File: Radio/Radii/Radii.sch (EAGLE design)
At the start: 14 parts, among them U2 LEV_SHIFT

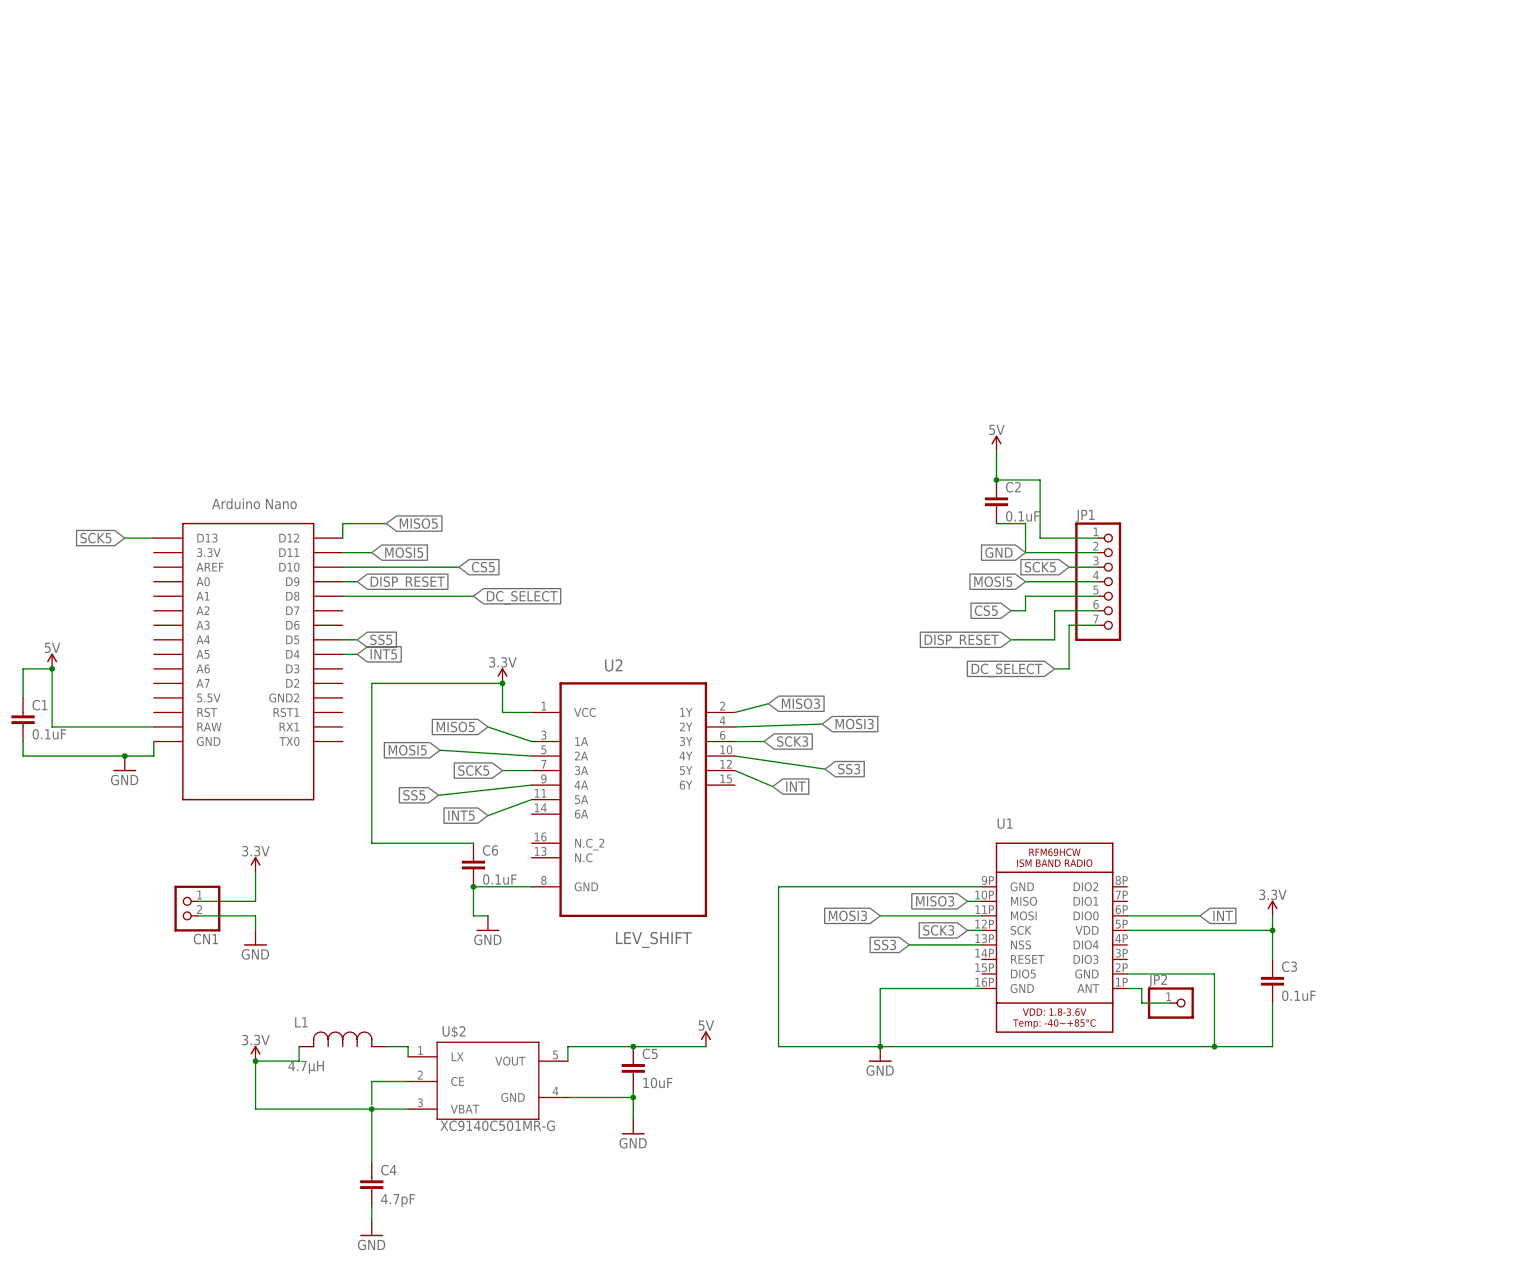
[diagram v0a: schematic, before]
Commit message: Radii Style Guide Changes
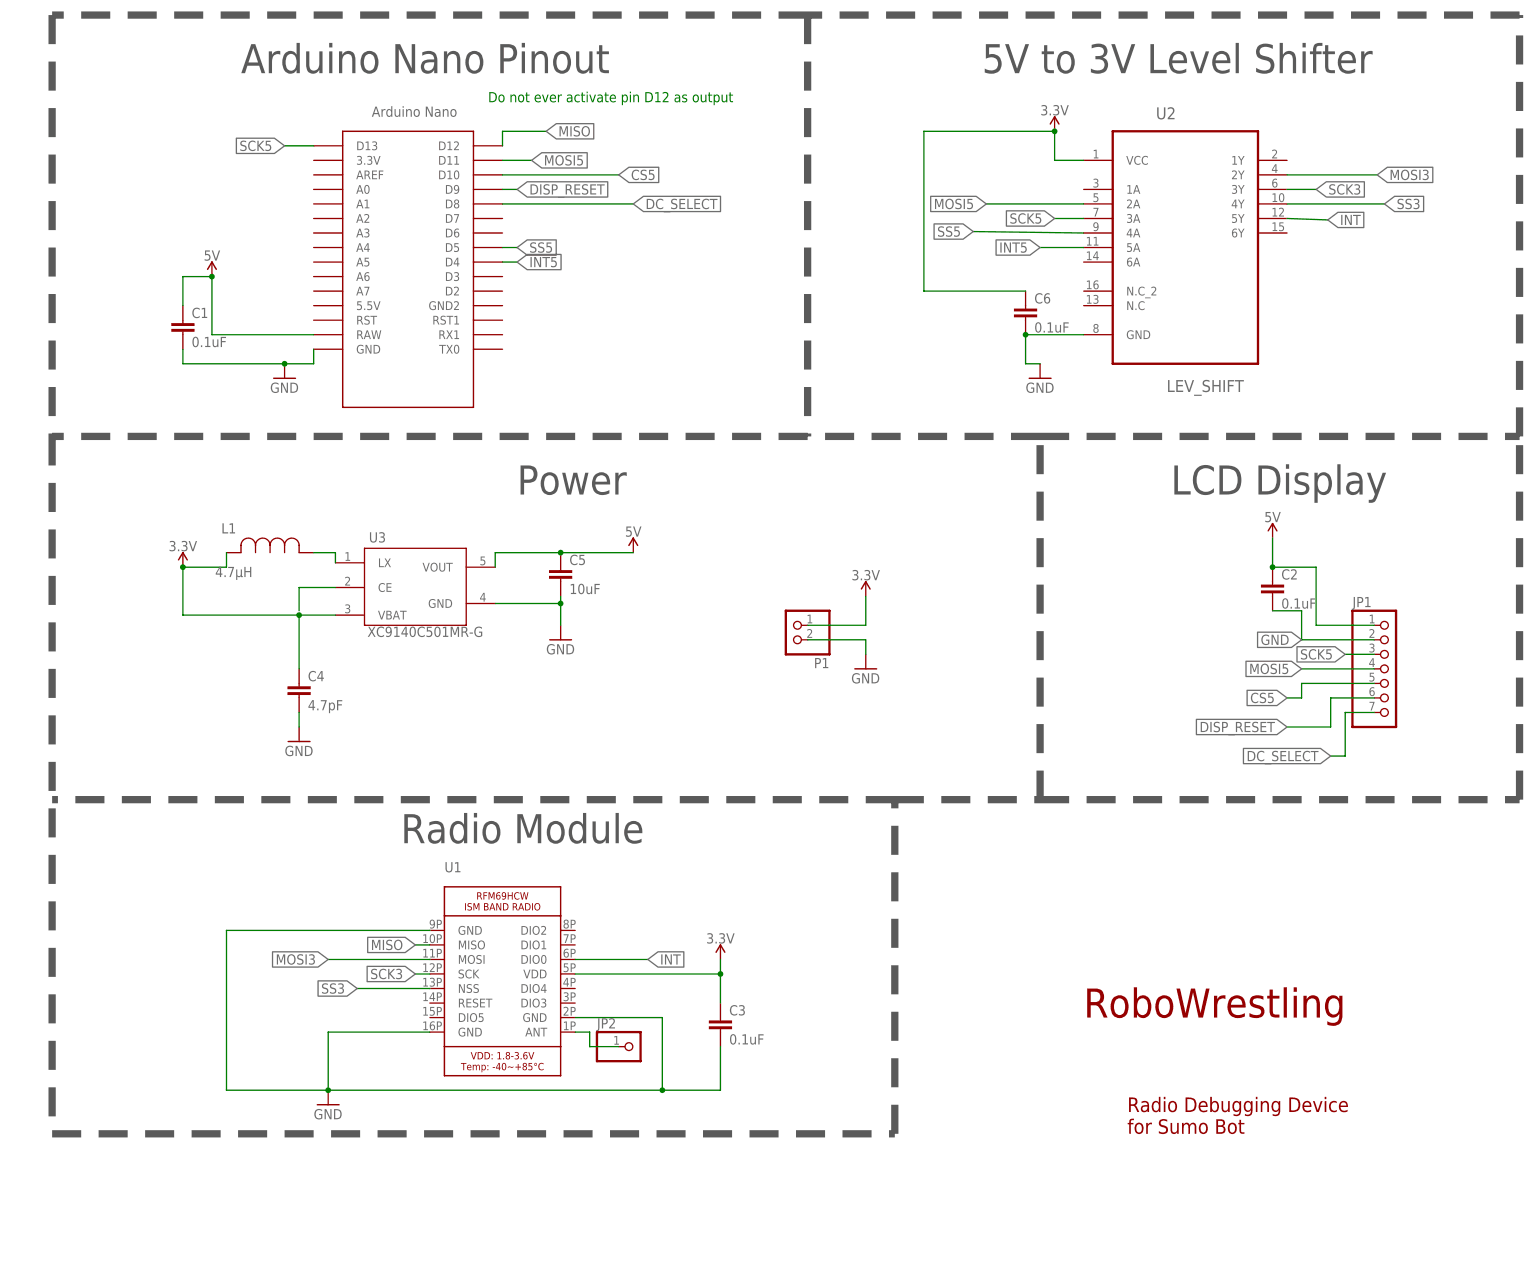
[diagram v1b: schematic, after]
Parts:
- removed CN1: (no value), adafruit:JST_2PIN-SMT-RA
- removed U$1: NANO, I'mRADIOactive:NANO
- removed U$2: XC9140C501MR-G, I'mRADIOactive:XC9140C501MR-G
- added P1: (no value), adafruit:JST_2PIN-SMT-RA
- added U3: XC9140C501MR-G, I'mRADIOactive:XC9140C501MR-G
- added U4: NANO, I'mRADIOactive:NANO
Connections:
- removed net MISO3: U1.MISO, U2.1Y
- removed net MISO5: U$1.D12, U2.1A
- new net MISO: U1.MISO, U4.D12
- net 3.3V: now also P1.2, U3.VBAT; no longer CN1.2, U$2.VBAT
- net 5V: now also U3.VOUT, U4.RAW; no longer U$1.RAW, U$2.VOUT
- net CS5: now also U4.D10; no longer U$1.D10
- net DC_SELECT: now also U4.D8; no longer U$1.D8
- net DISP_RESET: now also U4.D9; no longer U$1.D9
- net GND: now also P1.1, U3.GND, U4.GND; no longer CN1.1, U$1.GND, U$2.GND
- net INT5: now also U4.D4; no longer U$1.D4
- net MOSI5: now also U4.D11; no longer U$1.D11
- net N$1: now also U3.LX; no longer U$2.LX
- net N$2: now also U3.CE; no longer U$2.CE
- net SCK5: now also U4.D13; no longer U$1.D13
- net SS5: now also U4.D5; no longer U$1.D5
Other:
- note added: "5V to 3V Level Shifter"
- note added: "Arduino Nano Pinout"
- note added: "Do not ever activate pin D12 as output"
- note added: "LCD Display"
- note added: "Power"
- note added: "Radio Debugging Device for Sumo Bot"
- note added: "Radio Module"
- note added: "RoboWrestling"
- moved on the sheet: C1, C2, C3, C4, C5, C6, JP1, JP2, L1, U1, U2

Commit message: Changed to MCU
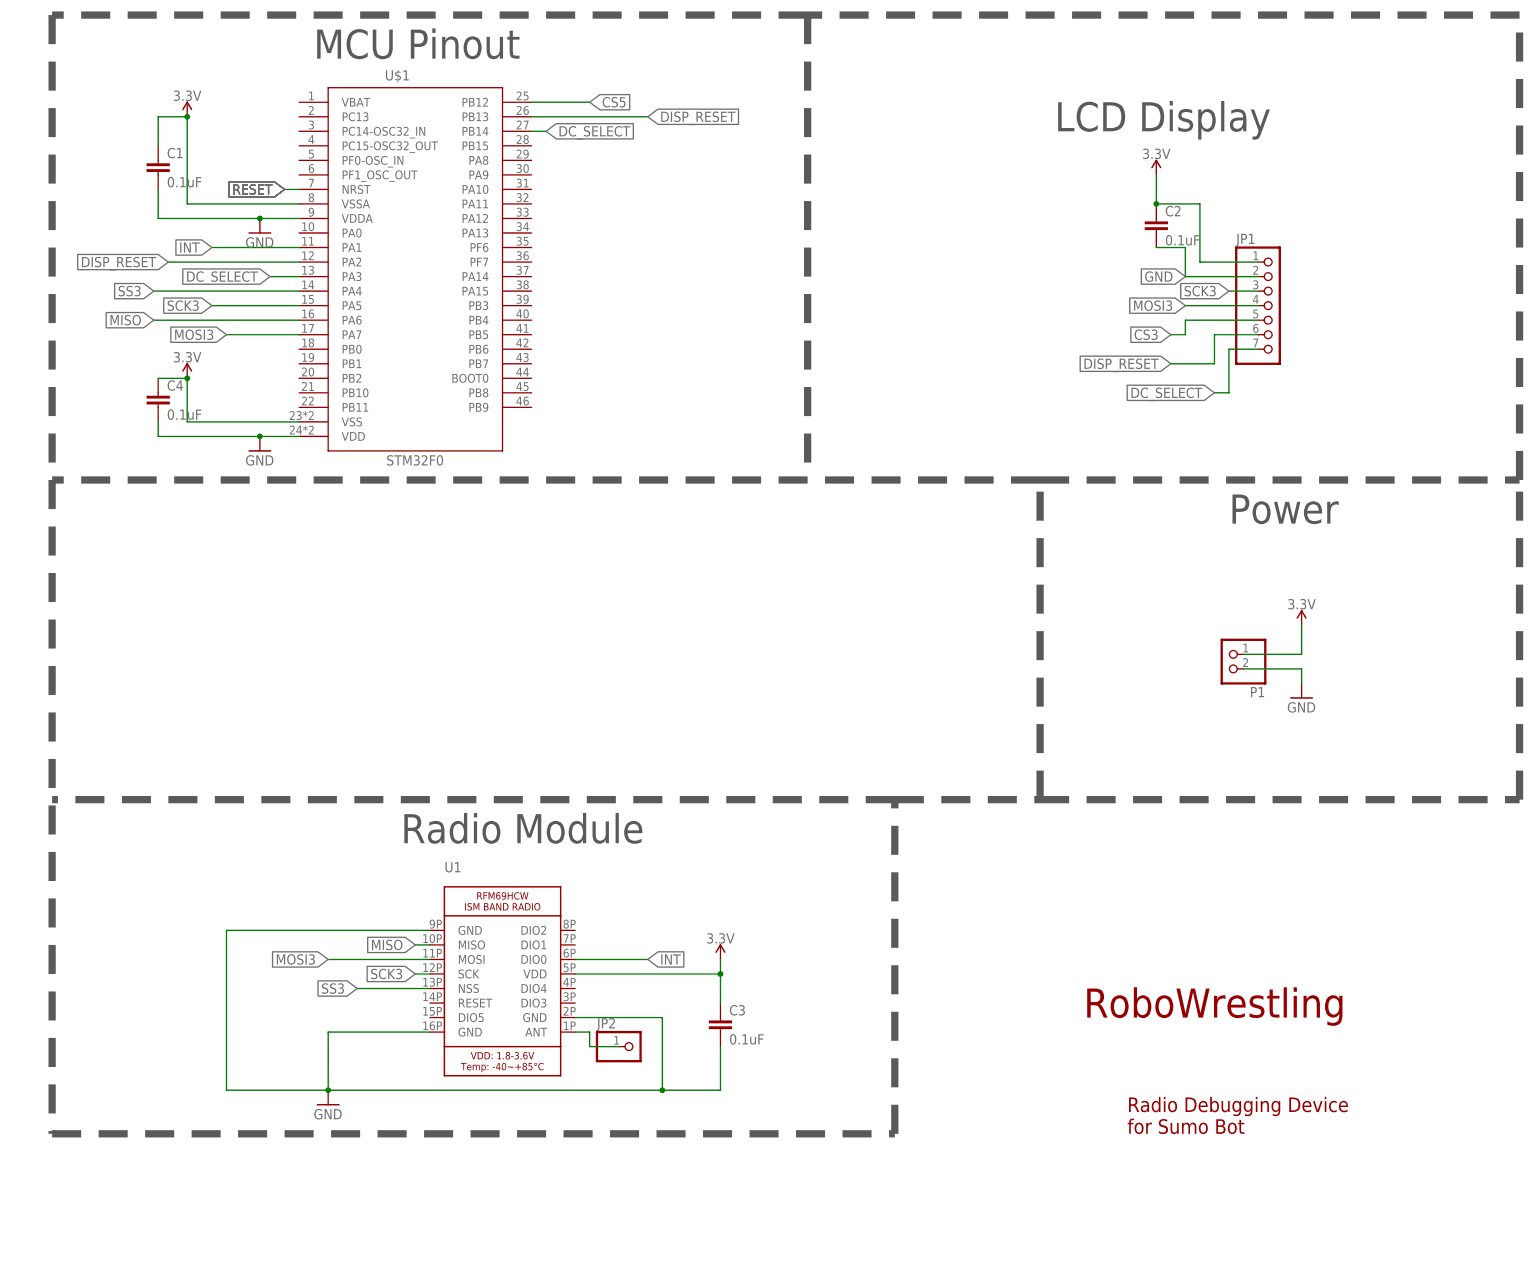
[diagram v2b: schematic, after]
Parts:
- removed C5: 10uF, SparkFun-Capacitors:10UF-0603-6.3V-20%
- removed C6: 0.1uF, SparkFun-Capacitors:0.1UF-0603-25V-(+80/-20%)
- removed L1: 4.7μH, I'mRADIOactive:SRN3015-4R7M
- removed U2: LEV_SHIFT, I'mRADIOactive:74HC4050D,653
- removed U3: XC9140C501MR-G, I'mRADIOactive:XC9140C501MR-G
- removed U4: NANO, I'mRADIOactive:NANO
- added U$1: STM32F0, I'mRADIOactive:STM32F0
- C4: value 4.7pF -> 0.1uF; device SparkFun-Capacitors:4.7PF-0603-50V-5% -> SparkFun-Capacitors:0.1UF-0603-25V-(+80/-20%)
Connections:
- removed net 5V: C1.1, C2.1, C5.1, JP1.1, U3.VOUT, U4.RAW
- removed net INT5: U2.5A, U4.D4
- removed net MOSI5: JP1.4, U2.2A, U4.D11
- removed net N$1: L1.1, U3.LX
- removed net N$2: U3.CE
- removed net SCK5: JP1.3, U2.3A, U4.D13
- removed net SS5: U2.4A, U4.D5
- new net CS3: JP1.5
- new net RESET: U$1.NRST
- net 3.3V: now also C1.1, C2.1, JP1.1, U$1.VSS, U$1.VSSA; no longer C6.1, L1.2, U2.VCC, U3.VBAT
- net CS5: now also U$1.PB12; no longer JP1.5, U4.D10
- net DC_SELECT: now also U$1.PA3, U$1.PB14; no longer U4.D8
- net DISP_RESET: now also U$1.PA2, U$1.PB13; no longer U4.D9
- net GND: now also U$1.VDD, U$1.VDDA; no longer C5.2, C6.2, U2.GND, U3.GND, U4.GND
- net INT: now also U$1.PA1; no longer U2.5Y
- net MISO: now also U$1.PA6; no longer U4.D12
- net MOSI3: now also JP1.4, U$1.PA7; no longer U2.2Y
- net SCK3: now also JP1.3, U$1.PA5; no longer U2.3Y
- net SS3: now also U$1.PA4; no longer U2.4Y
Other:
- note added: "MCU Pinout"
- note removed: "5V to 3V Level Shifter"
- note removed: "Arduino Nano Pinout"
- note removed: "Do not ever activate pin D12 as output"
- moved on the sheet: C1, C2, C4, JP1, P1
